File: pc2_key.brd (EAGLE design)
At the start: 100 x 34.9 mm, 51 parts

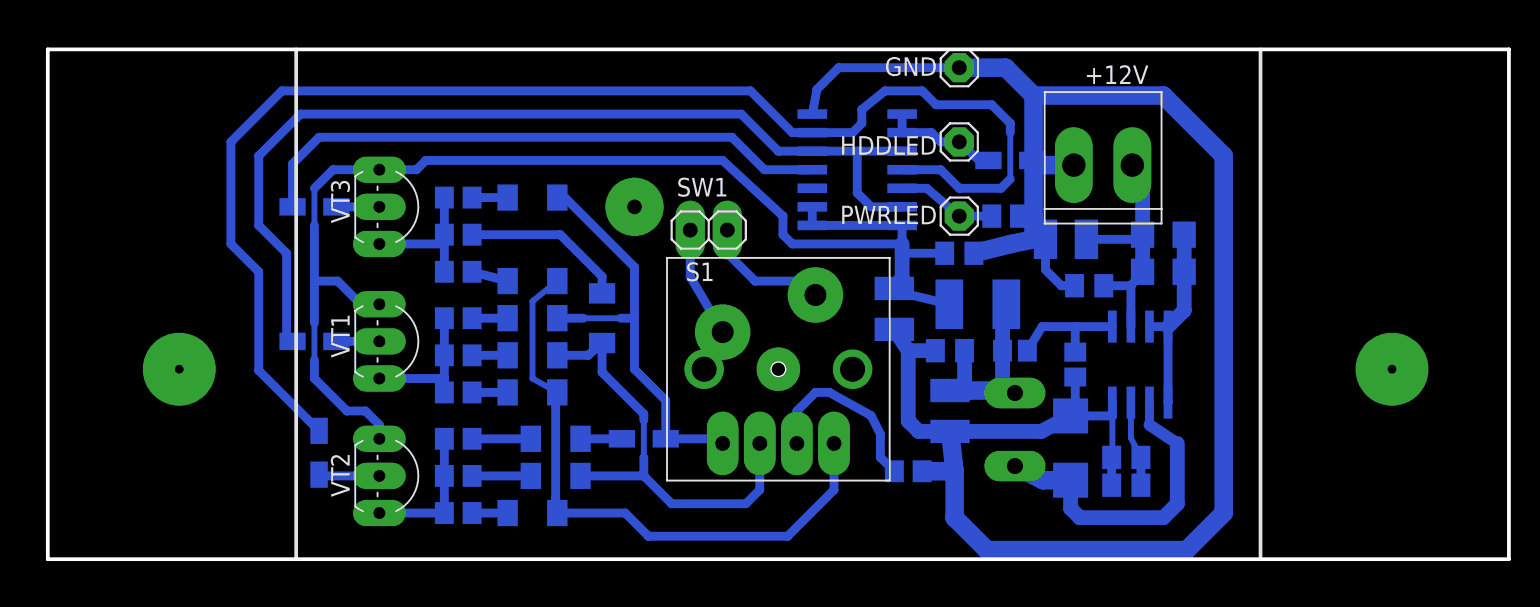
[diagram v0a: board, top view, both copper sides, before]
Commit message: 18
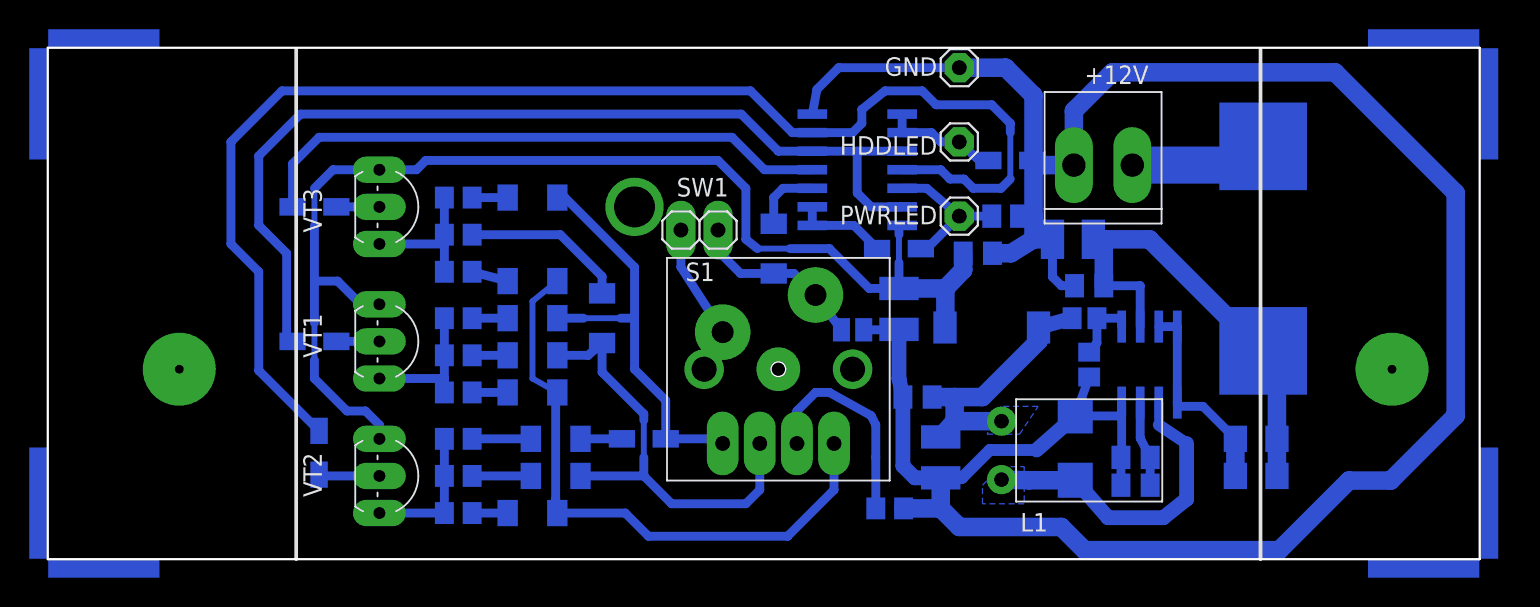
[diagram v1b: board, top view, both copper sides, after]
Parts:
- added 3VDB1: LL4148, diode:SOD80C
- added F1: (no value), fuse:SH32
- added J2: (no value), rcl:R1206W
- added SJ1: (no value), jumper:SJ
- added U$5, U$6, U$7, U$8: (no value), marks:ANGLE-SW-1
- C3, C5: value 10m -> 22m
- L1: device inductor-neosid:SD12K100 -> ct-pack:LH7X10MM
- L2: value (none) -> 10mkhn; device rcl:L1812 -> rcl:PIS2816
- moved J1 21.8 mm to (8.26, 8.26)
- moved R1A 15.3 mm to (32.7, -4.76), turned to 0 degrees
- moved R1B 15.3 mm to (32.7, -7.30), turned to 0 degrees
- moved L1 5.28 mm to (21.3, -5.56), flipped to the top, turned to 270 degrees
- moved R3 5.26 mm to (21.0, 3.49)
- moved C6 3.88 mm to (9.53, -1.91)
- moved C5 3.24 mm to (11.1, -6.03)
- moved RC1 2.84 mm to (7.62, -9.53)
- moved L2 1.85 mm to (14.6, 2.86), turned to 90 degrees
- moved C7 1.27 mm to (13.7, 7.94)
- moved R2 0.95 mm to (21.3, 0.32)
- moved C3A 0.64 mm to (24.4, -6.03)
- moved C3B 0.64 mm to (24.4, -7.94)
- moved SW1 0.63 mm to (-5.40, 9.53)
- moved DA1 0.63 mm to (25.4, 0.32)
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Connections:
- new net N$32: 3VDB1.C, DD1.3
- new net N$33: +12V.1, F1.P$1
- new net N$34: DD1.1, DD1.2, J1.2
- net +3V3: no longer DD1.1, DD1.2
- net GND: now also SJ1.1
- net N$19: now also L1.2; no longer L1.1
- net N$21: now also 3VDB1.A, SJ1.2
- net N$24: now also J2.2; no longer J1.2
- net N$29: now also L1.1; no longer L1.2
- net N$30: now also F1.P$2; no longer +12V.1
- net N$4: now also J2.1; no longer J1.1
- net PWRLED: now also J1.1
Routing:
- net GND: track 141.0 -> 173.0 mm
- net N$30: track 18.0 -> 32.7 mm
- net N$33: track 0.00 -> 10.2 mm
- net N$34: track 0.00 -> 6.36 mm
- net N$32: track 0.00 -> 4.70 mm
- net N$29: track 14.1 -> 18.5 mm
- net N$25: track 8.70 -> 4.78 mm
- net +3V3: track 88.2 -> 84.6 mm
- net PWRLED: track 6.84 -> 10.4 mm
- net N$21: track 8.80 -> 12.3 mm
- net N$23: track 12.6 -> 14.7 mm
- net N$3: track 13.3 -> 14.2 mm
- added copper zone on layer 16, net N$19
- added copper zone on layer 16, net N$29
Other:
- board size 100 x 34.9 mm -> 98 x 35 mm
